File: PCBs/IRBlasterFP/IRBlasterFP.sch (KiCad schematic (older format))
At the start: 5 parts, among them J1 Front Panel 2, U1 TSOP38238

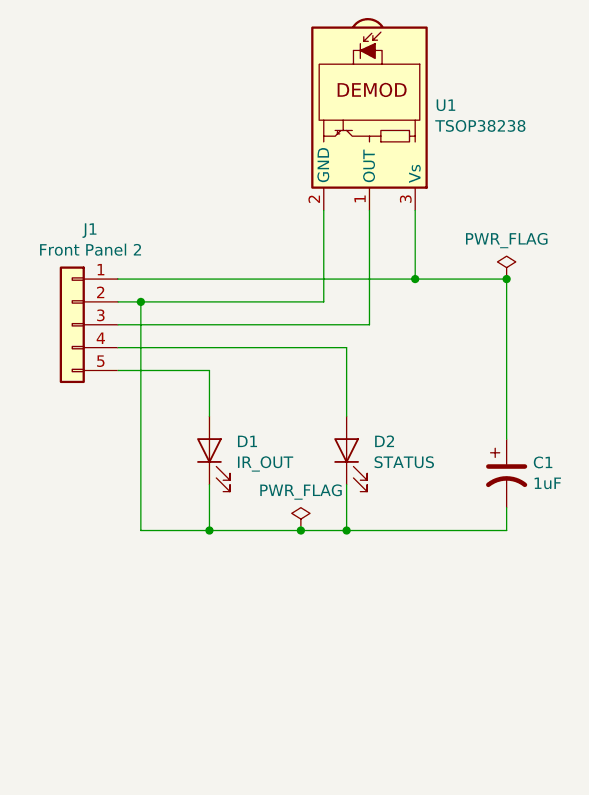
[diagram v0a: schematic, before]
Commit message: New designs
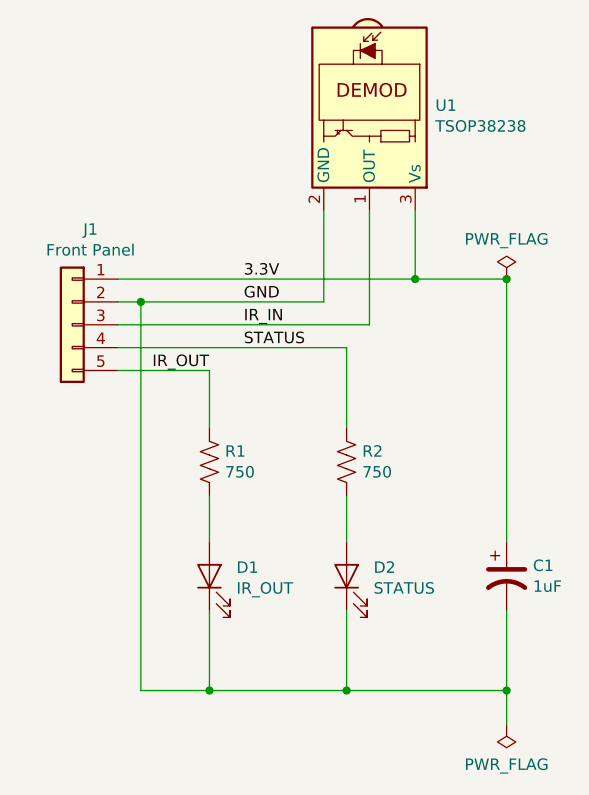
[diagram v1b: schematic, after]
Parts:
- added R1, R2: 750, Resistors_THT:R_Axial_DIN0204_L3.6mm_D1.6mm_P1.90mm_Vertical, symbol Device:R_US
- J1: value Front Panel 2 -> Front Panel
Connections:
- net IR_IN: now reaches J1.3 (Pin_3), U1.1 (OUT)
- net GND: now reaches C1.2, D1.1 (K), D2.1 (K), J1.2 (Pin_2), U1.2 (GND)
- net 3.3V: now reaches C1.1, J1.1 (Pin_1), U1.3 (Vs)
- net at D1.2 (A): now also R1.2; no longer J1.5 (Pin_5)
- net at D2.2 (A): now also R2.2; no longer J1.4 (Pin_4)
- new net IR_OUT: J1.5 (Pin_5), R1.1
- new net STATUS: J1.4 (Pin_4), R2.1
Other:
- moved on the sheet: D1, D2
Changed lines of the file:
@@
 L Device:LED D1
 U 1 1 5DBC6F3B
-P 5100 4550
-F 0 "D1" V 5138 4432 50  0000 R CNN
-F 1 "IR_OUT" V 5047 4432 50  0000 R CNN
-F 2 "LEDs:LED_D3.0mm" H 5100 4550 50  0001 C CNN
-F 3 "~" H 5100 4550 50  0001 C CNN
-F 4 "https://www.digikey.com/product-detail/en/broadcom-limited/HLMP-1700-B0002/516-1791-1-ND/1966497" H 5100 4550 50  0001 C CNN "DigiKey"
-	1    5100 4550
+P 5100 5100
+F 0 "D1" V 5138 4982 50  0000 R CNN
+F 1 "IR_OUT" V 5047 4982 50  0000 R CNN
+F 2 "LEDs:LED_D3.0mm" H 5100 5100 50  0001 C CNN
+F 3 "~" H 5100 5100 50  0001 C CNN
+F 4 "https://www.digikey.com/product-detail/en/broadcom-limited/HLMP-1700-B0002/516-1791-1-ND/1966497" H 5100 5100 50  0001 C CNN "DigiKey"
+	1    5100 5100
 	0    -1   -1   0
 $EndComp
@@
 L Device:LED D2
 U 1 1 5DBC71CC
-P 5700 4550
-F 0 "D2" V 5738 4432 50  0000 R CNN
-F 1 "STATUS" V 5647 4432 50  0000 R CNN
-F 2 "LEDs:LED_D3.0mm" H 5700 4550 50  0001 C CNN
-F 3 "~" H 5700 4550 50  0001 C CNN
-F 4 "https://www.digikey.com/product-detail/en/broadcom-limited/HLMP-1700-B0002/516-1791-1-ND/1966497" H 5700 4550 50  0001 C CNN "DigiKey"
-	1    5700 4550
+P 5700 5100
+F 0 "D2" V 5738 4982 50  0000 R CNN
+F 1 "STATUS" V 5647 4982 50  0000 R CNN
+F 2 "LEDs:LED_D3.0mm" H 5700 5100 50  0001 C CNN
+F 3 "~" H 5700 5100 50  0001 C CNN
+F 4 "https://www.digikey.com/product-detail/en/broadcom-limited/HLMP-1700-B0002/516-1791-1-ND/1966497" H 5700 5100 50  0001 C CNN "DigiKey"
+	1    5700 5100
 	0    -1   -1   0
 $EndComp
@@
 P 4500 4000
 F 0 "J1" H 4420 4417 50  0000 C CNN
-F 1 "Front Panel 2" H 4420 4326 50  0000 C CNN
+F 1 "Front Panel" H 4420 4326 50  0000 C CNN
 F 2 "Pin_Headers:Pin_Header_Straight_1x05_Pitch2.54mm" H 4500 4000 50  0001 C CNN
 F 3 "~" H 4500 4000 50  0001 C CNN
 	1    4500 4000
 	-1   0    0    -1
-$EndComp
-$Comp
-L Device:CP1 C1
-U 1 1 5DBC7797
-P 6400 4650
-F 0 "C1" H 6515 4696 50  0000 L CNN
-F 1 "1uF" H 6515 4605 50  0000 L CNN
-F 2 "Capacitors_THT:CP_Radial_D5.0mm_P2.50mm" H 6400 4650 50  0001 C CNN
-F 3 "~" H 6400 4650 50  0001 C CNN
-	1    6400 4650
-	1    0    0    -1
 $EndComp
 $Comp
@@
 $EndComp
 Wire Wire Line
-	4700 3900 4800 3900
-Wire Wire Line
 	5600 3900 5600 3500
 Wire Wire Line
 	4700 4100 5700 4100
 Wire Wire Line
-	5700 4100 5700 4400
+	5100 5250 5100 5600
 Wire Wire Line
-	5100 4700 5100 4900
+	5700 5600 5700 5250
 Wire Wire Line
-	5100 4900 5500 4900
+	5700 5600 6400 5600
 Wire Wire Line
-	5700 4900 5700 4700
+	6400 5600 6400 5250
+Connection ~ 5700 5600
 Wire Wire Line
-	5700 4900 6400 4900
-Wire Wire Line
-	6400 4900 6400 4800
-Connection ~ 5700 4900
-Wire Wire Line
-	6400 4500 6400 3800
-Wire Wire Line
-	4800 3900 4800 4900
-Wire Wire Line
-	4800 4900 5100 4900
-Connection ~ 4800 3900
-Wire Wire Line
-	4800 3900 5600 3900
-Connection ~ 5100 4900
-Connection ~ 6400 3800
+	4800 5600 5100 5600
+Connection ~ 5100 5600
 Wire Wire Line
 	6000 3500 6000 3800
@@
 Wire Wire Line
 	5800 3500 5800 4000
-$Comp
-L power:PWR_FLAG #FLG0102
-U 1 1 5DC1E0EE
-P 5500 4900
-F 0 "#FLG0102" H 5500 4975 50  0001 C CNN
-F 1 "PWR_FLAG" H 5500 5074 50  0000 C CNN
-F 2 "" H 5500 4900 50  0001 C CNN
-F 3 "~" H 5500 4900 50  0001 C CNN
-	1    5500 4900
-	1    0    0    -1
-$EndComp
-Connection ~ 5500 4900
-Wire Wire Line
-	5500 4900 5700 4900
 Wire Wire Line
 	4700 4200 5100 4200
 Wire Wire Line
-	5100 4200 5100 4400
+	4700 4000 5800 4000
+Text Label 5250 3800 0    50   ~ 0
+3.3V
+Text Label 5250 3900 0    50   ~ 0
+GND
+Text Label 5250 4000 0    50   ~ 0
+IR_IN
+Text Label 5250 4100 0    50   ~ 0
+STATUS
+Text Label 4850 4200 0    50   ~ 0
+IR_OUT
+$Comp
+L Device:CP1 C1
+U 1 1 5DC1CE96
+P 6400 5100
+F 0 "C1" H 6515 5146 50  0000 L CNN
+F 1 "1uF" H 6515 5055 50  0000 L CNN
+F 2 "Capacitors_THT:CP_Radial_D5.0mm_P2.50mm" H 6400 5100 50  0001 C CNN
+F 3 "~" H 6400 5100 50  0001 C CNN
+	1    6400 5100
+	1    0    0    -1
+$EndComp
+$Comp
+L Device:R_US R1
+U 1 1 5DC1D2DC
+P 5100 4600
+F 0 "R1" H 5168 4646 50  0000 L CNN
+F 1 "750" H 5168 4555 50  0000 L CNN
+F 2 "Resistors_THT:R_Axial_DIN0204_L3.6mm_D1.6mm_P1.90mm_Vertical" V 5140 4590 50  0001 C CNN
+F 3 "~" H 5100 4600 50  0001 C CNN
+	1    5100 4600
+	1    0    0    -1
+$EndComp
+$Comp
+L Device:R_US R2
+U 1 1 5DC1D326
+P 5700 4600
+F 0 "R2" H 5768 4646 50  0000 L CNN
+F 1 "750" H 5768 4555 50  0000 L CNN
+F 2 "Resistors_THT:R_Axial_DIN0204_L3.6mm_D1.6mm_P1.90mm_Vertical" V 5740 4590 50  0001 C CNN
+F 3 "~" H 5700 4600 50  0001 C CNN
+	1    5700 4600
+	1    0    0    -1
+$EndComp
 Wire Wire Line
-	4700 4000 5800 4000
+	4700 3900 4800 3900
+Wire Wire Line
+	4800 3900 4800 5600
+Connection ~ 4800 3900
+Wire Wire Line
+	4800 3900 5600 3900
+Wire Wire Line
+	6400 3800 6400 4950
+Connection ~ 6400 3800
+Wire Wire Line
+	5100 5600 5700 5600
+Wire Wire Line
+	6400 5750 6400 5600
+Connection ~ 6400 5600
+Wire Wire Line
+	5100 4450 5100 4200
+Wire Wire Line
+	5700 4100 5700 4450
+Wire Wire Line
+	5700 4750 5700 4950
+Wire Wire Line
+	5100 4750 5100 4950
+$Comp
+L power:PWR_FLAG #FLG0102
+U 1 1 5DC1EE70
+P 6400 5750
+F 0 "#FLG0102" H 6400 5825 50  0001 C CNN
+F 1 "PWR_FLAG" H 6400 5924 50  0000 C CNN
+F 2 "" H 6400 5750 50  0001 C CNN
+F 3 "~" H 6400 5750 50  0001 C CNN
+	1    6400 5750
+	-1   0    0    1
+$EndComp
 $EndSCHEMATC
